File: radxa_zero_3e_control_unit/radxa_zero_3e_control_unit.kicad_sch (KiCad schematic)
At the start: 44 parts, among them J14 DebugUART, J16 Malibotti, J17 Robot, J18 STLINK_V3_MINIE, J19 IO, J21 STDC14, J22 USB STM32, J23 IO, J24 IO, J25 IO, J28 RADXA I2C, J29 RADXA GPIO, J3 TOF3, J4 TOF2, J5 TOF1, J6 TOF1, U2 STM32G431RBTx, X1 Radxa Zero 3E

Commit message: Udated control unit pcb
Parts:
- removed J17: Robot, Connector_JST:JST_XH_B4B-XH-A_1x04_P2.50mm_Vertical, symbol Connector_Generic:Conn_01x04
- removed J18: STLINK_V3_MINIE, Connector_IDC:IDC-Header_2x05_P2.54mm_Vertical, symbol Connector_Generic:Conn_02x05_Odd_Even
- removed J19: IO, Connector_JST:JST_XH_S5B-XH-A-1_1x05_P2.50mm_Horizontal, symbol Connector_Generic:Conn_01x05
- removed J23, J24, J25: IO, Connector_JST:JST_XH_B6B-XH-A_1x06_P2.50mm_Vertical, symbol Connector_Generic:Conn_01x06
- removed J28: RADXA I2C, Connector_JST:JST_XH_B4B-XH-A_1x04_P2.50mm_Vertical, symbol Connector_Generic:Conn_01x04
- removed J29: RADXA GPIO, Connector_JST:JST_XH_B4B-XH-A_1x04_P2.50mm_Vertical, symbol Connector_Generic:Conn_01x04
- added C41: u1, Capacitor_SMD:C_0402_1005Metric, symbol Device:C
- added H3, H4: M2,5, MountingHole:MountingHole_2.7mm, symbol Mechanical:MountingHole
- added J11: Raspberry_Pi_5, liebler_MODULES:RasPi5, symbol Connector:Raspberry_Pi_4
- added J12: CAN, liebler_CONN:JST_XH_B3B-XH-A_1x03_P2.50mm_Vertical_smaller, symbol Connector_Generic:Conn_01x03
- added J30: LightBarrier1, liebler_CONN:JST_XH_B3B-XH-A_1x03_P2.50mm_Vertical_smaller, symbol Connector_Generic:Conn_01x03
- added J31: LightBarrier2, liebler_CONN:JST_XH_B3B-XH-A_1x03_P2.50mm_Vertical_smaller, symbol Connector_Generic:Conn_01x03
- added J32: LightBarrier3, liebler_CONN:JST_XH_B3B-XH-A_1x03_P2.50mm_Vertical_smaller, symbol Connector_Generic:Conn_01x03
- added J33: PressureTransducer, liebler_CONN:JST_XH_B3B-XH-A_1x03_P2.50mm_Vertical_smaller, symbol Connector_Generic:Conn_01x03
- added JP2, JP3, JP4: 5-24, Jumper:SolderJumper-3_P1.3mm_Open_RoundedPad1.0x1.5mm_NumberLabels, symbol Jumper:SolderJumper_3_Open
- added M1: W5500_mini, liebler_MODULES:W5500-mini, symbol liebler_MODULES:W5500_mini
- added M2: FanMech, liebler_MECH:FAN2507, symbol Motor:Fan
- added M3: FanElek, Connector_JST:JST_XH_B2B-XH-A_1x02_P2.50mm_Vertical, symbol Motor:Fan
- added R32, R34, R35: 10k, Resistor_SMD:R_0402_1005Metric, symbol Device:R
- added R36: 1k, Resistor_SMD:R_0402_1005Metric, symbol Device:R
- added U7: SIT3051TK, Package_DFN_QFN:DFN-8-1EP_3x3mm_P0.65mm_EP1.55x2.4mm, symbol liebler_SEMICONDUCTORS:SIT3051TK
- C12, C15, C16, C17, C18, C19, C9: footprint Capacitor_SMD:C_0201_0603Metric -> Capacitor_SMD:C_0402_1005Metric
- H6: footprint MountingHole:MountingHole_3.2mm_M3 -> MountingHole:MountingHole_2.7mm
- J16: footprint liebler_CONN:JST_XH_S4B-XH-A-1_1x04_P2.50mm_Horizontal_SmallerCourtyard -> liebler_CONN:JST_XH_B4B-XH-A_1x04_P2.50mm_Vertical_smaller
- J3, J4, J5: footprint Connector_JST:JST_XH_S5B-XH-A-1_1x05_P2.50mm_Horizontal -> liebler_CONN:JST_XH_B5B-XH-A_1x05_P2.50mm_Vertical_smaller
- J6: value TOF1 -> RGB; footprint Connector_JST:JST_XH_S5B-XH-A-1_1x05_P2.50mm_Horizontal -> liebler_CONN:JST_XH_B5B-XH-A_1x05_P2.50mm_Vertical_smaller
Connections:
- net HX711_CLK is gone; now on net INT_TOF1: U2.54 (PC12)
- net IO2 is gone; now on net INT_TOF2: U2.58 (PB5)
- net IO3 is gone; now on net INT_RGB: U2.55 (PD2)
- net PB13 is gone; now on net STEPPER_EN: U2.35 (PB13)
- net PC15 is gone; now on net INT_TOF3: U2.4 (PC15)
- net +3V3: now also C41.1, M1.10 (3V3), M1.11 (3V3), U7.3 (VCC)
- net +5V: now also J16.4 (Pin_4), J33.2 (Pin_2), JP2.1 (A), JP3.1 (A), JP4.1 (A), M3.1 (+); no longer J16.1 (Pin_1)
- net GND: now also J16.3 (Pin_3), C41.2, J12.2 (Pin_2), J30.3 (Pin_3), J31.3 (Pin_3), J32.3 (Pin_3), J33.3 (Pin_3), M1.1 (GND), M1.12 (GND), M1.2 (GND), M3.2 (-), R34.1, R35.1, U7.2 (GND), U7.9 (PAD); no longer J16.2 (Pin_2)
- net INT_RGB: no longer X1.15 (G3B0)
- net INT_TOF1: now also J5.3 (Pin_3); no longer J4.3 (Pin_3), U2.13 (PA1)
- net INT_TOF2: now also J4.3 (Pin_3); no longer J5.3 (Pin_3), U2.12 (PA0)
- net INT_TOF3: no longer U2.2 (PC13)
- net SCL: no longer J6.1 (Pin_1)
- net SDA: no longer J6.2 (Pin_2)
- net SPI1_MISO: now also M1.7 (MISO)
- net SPI1_MOSI: now also M1.3 (MOSI)
- net SPI1_NSS: now also M1.5 (~{CS}[PU])
- net SPI1_SCK: now also M1.4 (SCLK)
- net STEPPER_EN: no longer U2.42 (PA8)
- net USB_VSENSE: now also U2.42 (PA8); no longer U2.6 (PF1)
- net at X1.13 (G3A2/-/-/I2S3_MCLK): no longer JP1.2 (B)
- net STM32_BOOT_CAN_RX: now reaches X1.38 (G3A6/-/-/-/I3S_SDI)
- net STM32_BOOT_CAN_RX: now also U2.61 (PB8), R36.2
- net Compressor_PWM: no longer names the net of X1.24 (G4C6/S3_CS0/PWM13/U9R/I3S_SDI)
- net Conveyor_PWM: no longer names the net of X1.7 (G3C4/-/-/PWM14_M0)
- net G1A4: no longer names the net of X1.37 (G1A4/-/I1S_SCLK)
- net G3A4: no longer names the net of X1.35 (G3A4/-/I3S_LRCK)
- net HX711_DATA renamed ROBOT_U4R
- net I5C_C: no longer names the net of X1.29 (G3B3/-/-/I5C_SCL)
- net I5C_D: no longer names the net of X1.31 (G3B4/-/-/I5C_SSDA)
- net IO1 renamed CAN_TX
- net CAN_TX: now also U7.4 (R)
- net IO4 renamed ROBOT_U4T
- net MALIBOTTI_RXD: no longer names the net of X1.5 (G1A1/U3T/PU!)
- net MALIBOTTI_RXD: no longer J16.3 (Pin_3)
- net MALIBOTTI_TXD: no longer names the net of X1.3 (G1A0/U3R/PU!)
- net MALIBOTTI_TXD: no longer J16.4 (Pin_4)
- net PB12 renamed ADC1_IN11
- net PC14 renamed LightBarrier2
- net LightBarrier2: now also J31.1 (Pin_1)
- net ROBOT_RXD: no longer names the net of X1.18 (G3B2/U4T/PWM9)
- net ROBOT_TXD: no longer names the net of X1.16 (G3B1/U4R/PWM8)
- net STM32_BOOT: no longer names the net of X1.12 (G3A3)
- net STM32_BOOT: no longer U2.61 (PB8)
- net Stepper1_Dir renamed VALVE
- net Stepper1_Step renamed STEPPER1_DIR
- net Stepper2_Dir renamed ADC2_12
- net Stepper2_Step renamed STEPPER1_STEP
- net T15C1 renamed HX711_SPI2_MISO
- net T15C2 renamed HX711_SPI2_MOSI
- net T1C1-LU1R renamed MALIBOTTI_U1R
- net MALIBOTTI_U1R: now also J16.1 (Pin_1)
- net T1C2-LU1T renamed MALIBOTTI_U1T
- net MALIBOTTI_U1T: now also J16.2 (Pin_2)
- net T1C3 renamed PRESSURE_ADC
- net PRESSURE_ADC: now also R32.1, R34.2
- net T1C4 renamed W5500_IRQ
- net W5500_IRQ: now also M1.6 (~{INT}[PU])
- net T8C1 renamed STEPPER2_DIR_T3C1_T8C1
- net T8C2 renamed STEPPER2_STEP_T3C2_T8C2
- net Valve: no longer names the net of X1.36 (G3A7)
- net Valve: now also JP1.2 (B)
- net i1c renamed I2C2_SCL
- net i1d renamed I2C2_SDA
- net i2c renamed I2C1_SCL
- net I2C1_SCL: now also J6.1 (Pin_1), U2.51 (PA15); no longer U2.40 (PC8)
- net i2d renamed I2C1_SDA
- net I2C1_SDA: now also J6.2 (Pin_2), U2.60 (PB7); no longer U2.41 (PC9)
- net i3c renamed I2C3_SCL
- net I2C3_SCL: now also U2.40 (PC8); no longer U2.51 (PA15)
- net i3d renamed I2C3_SDA
- net I2C3_SDA: now also U2.41 (PC9); no longer U2.60 (PB7)
- new net: J30.2 (Pin_2), JP2.2 (C)
- new net: J32.2 (Pin_2), JP4.2 (C)
- new net: J31.2 (Pin_2), JP3.2 (C)
- new net: R35.2, U7.8 (Rs)
- new net: R36.1, U7.1 (D)
- new net: J33.1 (Pin_1), R32.2
- new net: J11.1 (3V3), J11.17 (3V3)
- new net: J11.14 (GND), J11.20 (GND), J11.25 (GND), J11.30 (GND), J11.34 (GND), J11.39 (GND), J11.6 (GND), J11.9 (GND)
- new net: J11.2 (5V), J11.4 (5V)
- new net +24V: JP2.3 (B), JP3.3 (B), JP4.3 (B)
- new net CANH: J12.1 (Pin_1), U7.7 (CANH)
- new net CANL: J12.3 (Pin_3), U7.6 (CANL)
- new net COMPRESSOR_T2C1: U2.12 (PA0)
- new net CONVEYOR_T2C2: U2.13 (PA1)
- new net LightBarrier1: J30.1 (Pin_1), U2.6 (PF1)
- new net LightBarrier3: J32.1 (Pin_1), U2.2 (PC13)
- no-connect marks 11 -> 9
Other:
- moved on the sheet: JP1

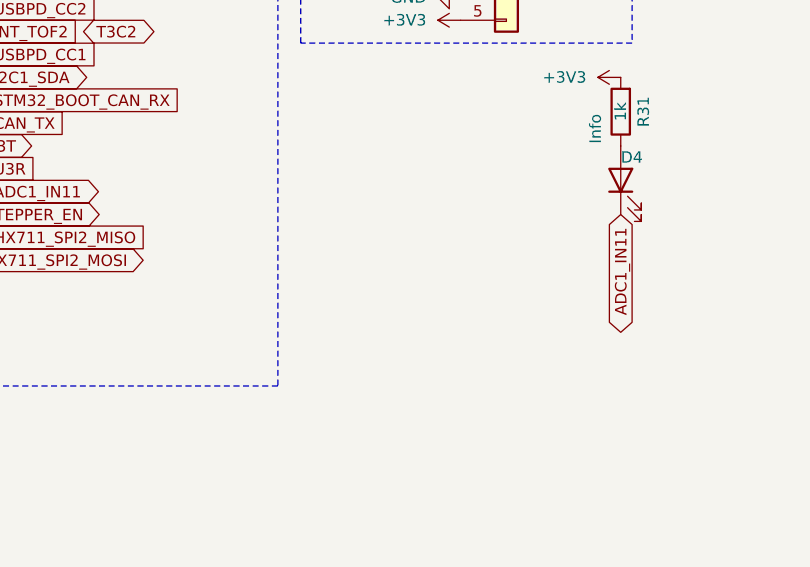
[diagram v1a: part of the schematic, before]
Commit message: Sigmoid Stepper
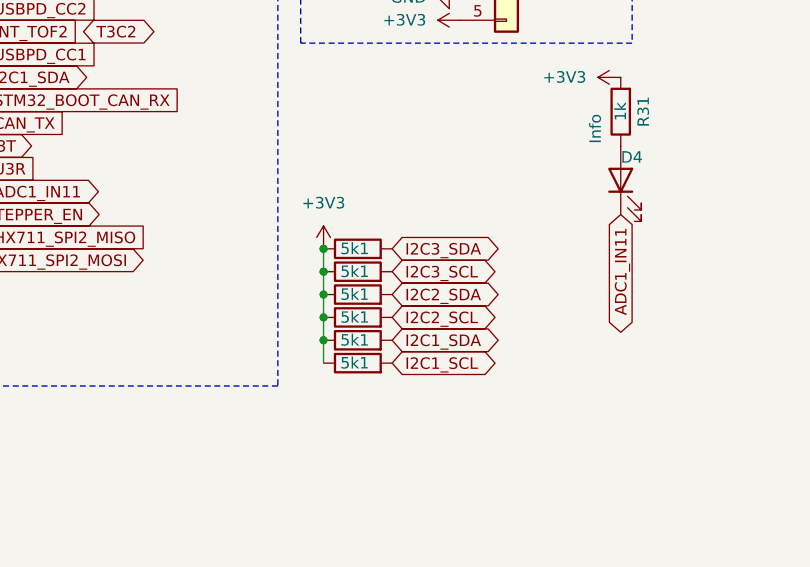
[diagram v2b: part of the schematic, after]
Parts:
- added R38, R39, R40, R41, R42, R43: 5k1, Resistor_SMD:R_0201_0603Metric, symbol Device:R
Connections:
- net +3V3: now also R38.1, R39.1, R40.1, R41.1, R42.1, R43.1
- net I2C1_SCL: now also R43.2
- net I2C1_SDA: now also R42.2
- net I2C2_SCL: now also R41.2
- net I2C2_SDA: now also R40.2
- net I2C3_SCL: now also R39.2
- net I2C3_SDA: now also R38.2
